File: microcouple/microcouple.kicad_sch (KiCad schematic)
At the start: 4 parts, among them J1 LiPo Battery, P1 USB_C_Plug

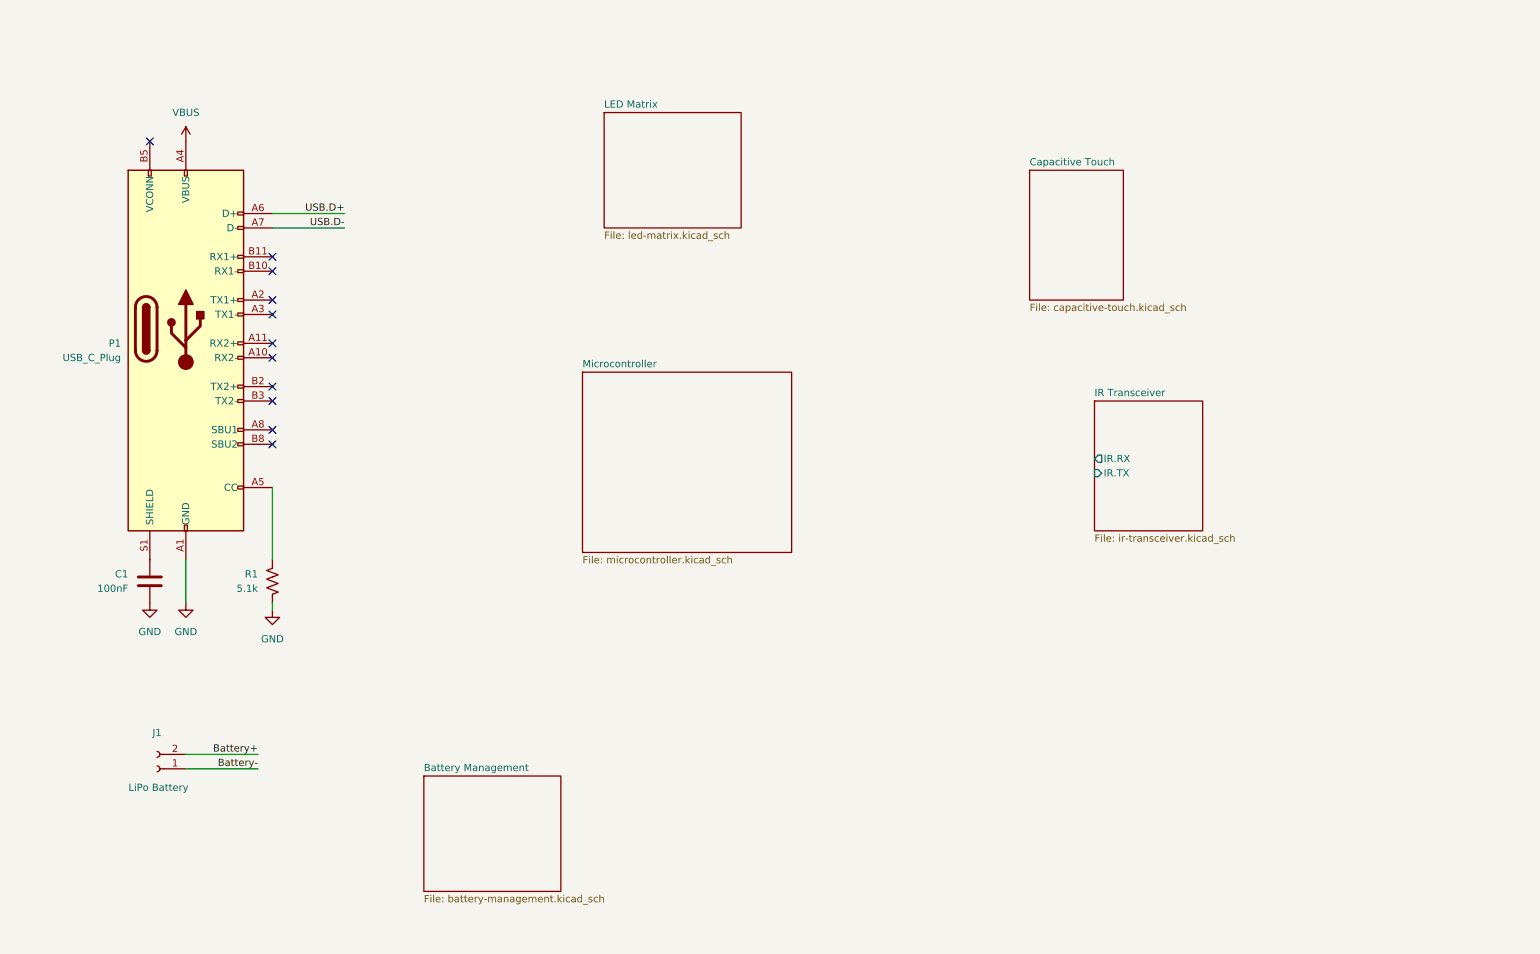
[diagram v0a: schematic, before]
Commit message: Finalize battery management
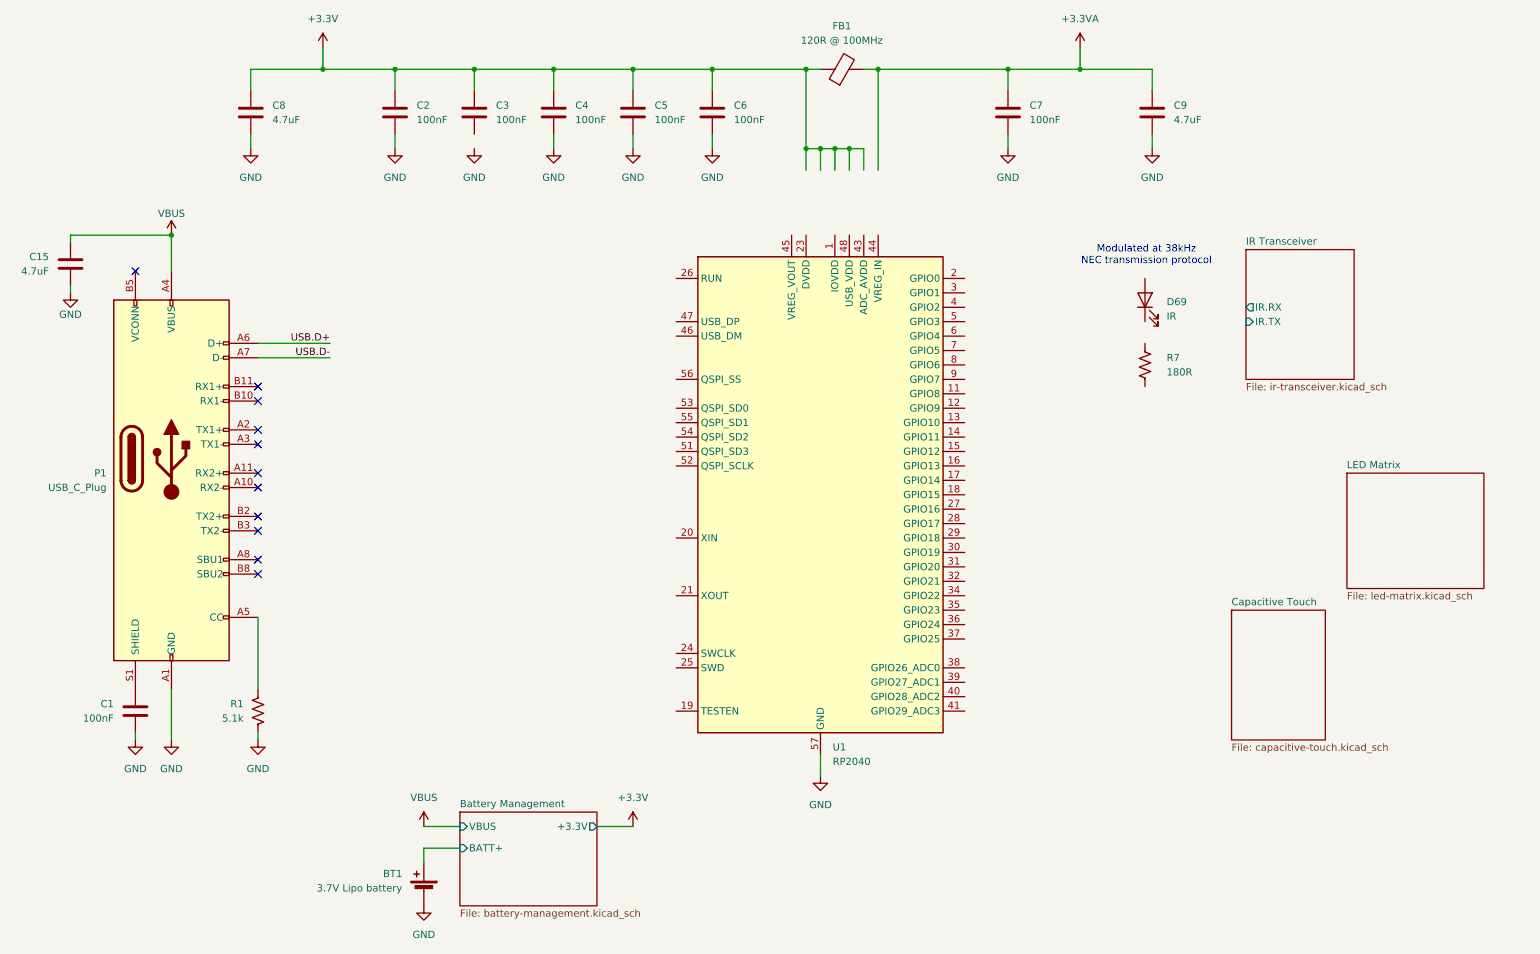
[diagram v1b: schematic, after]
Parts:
- removed J1: LiPo Battery, Connector_JST:JST_PH_S2B-PH-K_1x02_P2.00mm_Horizontal, symbol Connector:Conn_01x02_Socket
- added BT1: 3.7V Lipo battery, Connector_JST:JST_PH_S2B-PH-K_1x02_P2.00mm_Horizontal, symbol Device:Battery_Cell
- added C15, C8, C9: 4.7uF, Capacitor_SMD:C_0805_2012Metric_Pad1.18x1.45mm_HandSolder, symbol Device:C
- added C2, C3, C4, C5, C6, C7: 100nF, Capacitor_SMD:C_0805_2012Metric_Pad1.18x1.45mm_HandSolder, symbol Device:C
- added D69: IR, LED_THT:LED_D5.0mm_Horizontal_O1.27mm_Z3.0mm_Clear, symbol Device:LED
- added FB1: 120R @ 100MHz, Inductor_SMD:L_0805_2012Metric_Pad1.15x1.40mm_HandSolder, symbol Device:FerriteBead
- added R7: 180R, Resistor_SMD:R_0805_2012Metric_Pad1.20x1.40mm_HandSolder, symbol Device:R_US
- added U1: RP2040, Package_DFN_QFN:QFN-56-1EP_7x7mm_P0.4mm_EP3.2x3.2mm, symbol MCU_RaspberryPi:RP2040
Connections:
- net GND: now also BT1.2 (-), C15.2, C2.2, C4.2, C5.2, C6.2, C7.2, C8.2, C9.2, U1.57 (GND)
- net VBUS: now also C15.1
- new net: U1.1 (IOVDD), U1.10 (IOVDD), U1.22 (IOVDD), U1.33 (IOVDD), U1.42 (IOVDD), U1.49 (IOVDD)
- new net: U1.23 (DVDD), U1.50 (DVDD)
- new net +3.3V: C2.1, C3.1, C4.1, C5.1, C6.1, C8.1, FB1.1
- new net +3.3VA: C7.1, C9.1, FB1.2
- new net Battery Management/BATT+: BT1.1 (+)
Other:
- removed sheet Microcontroller
- sheet Battery Management ports: added +3.3V, BATT+, VBUS; removed none
- note added: "Modulated at 38kHz NEC transmission protocol"
- moved on the sheet: C1, P1, R1
